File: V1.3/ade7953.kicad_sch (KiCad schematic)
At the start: 57 parts, among them U2 ADE7953xCP, Y1 3.58MHz

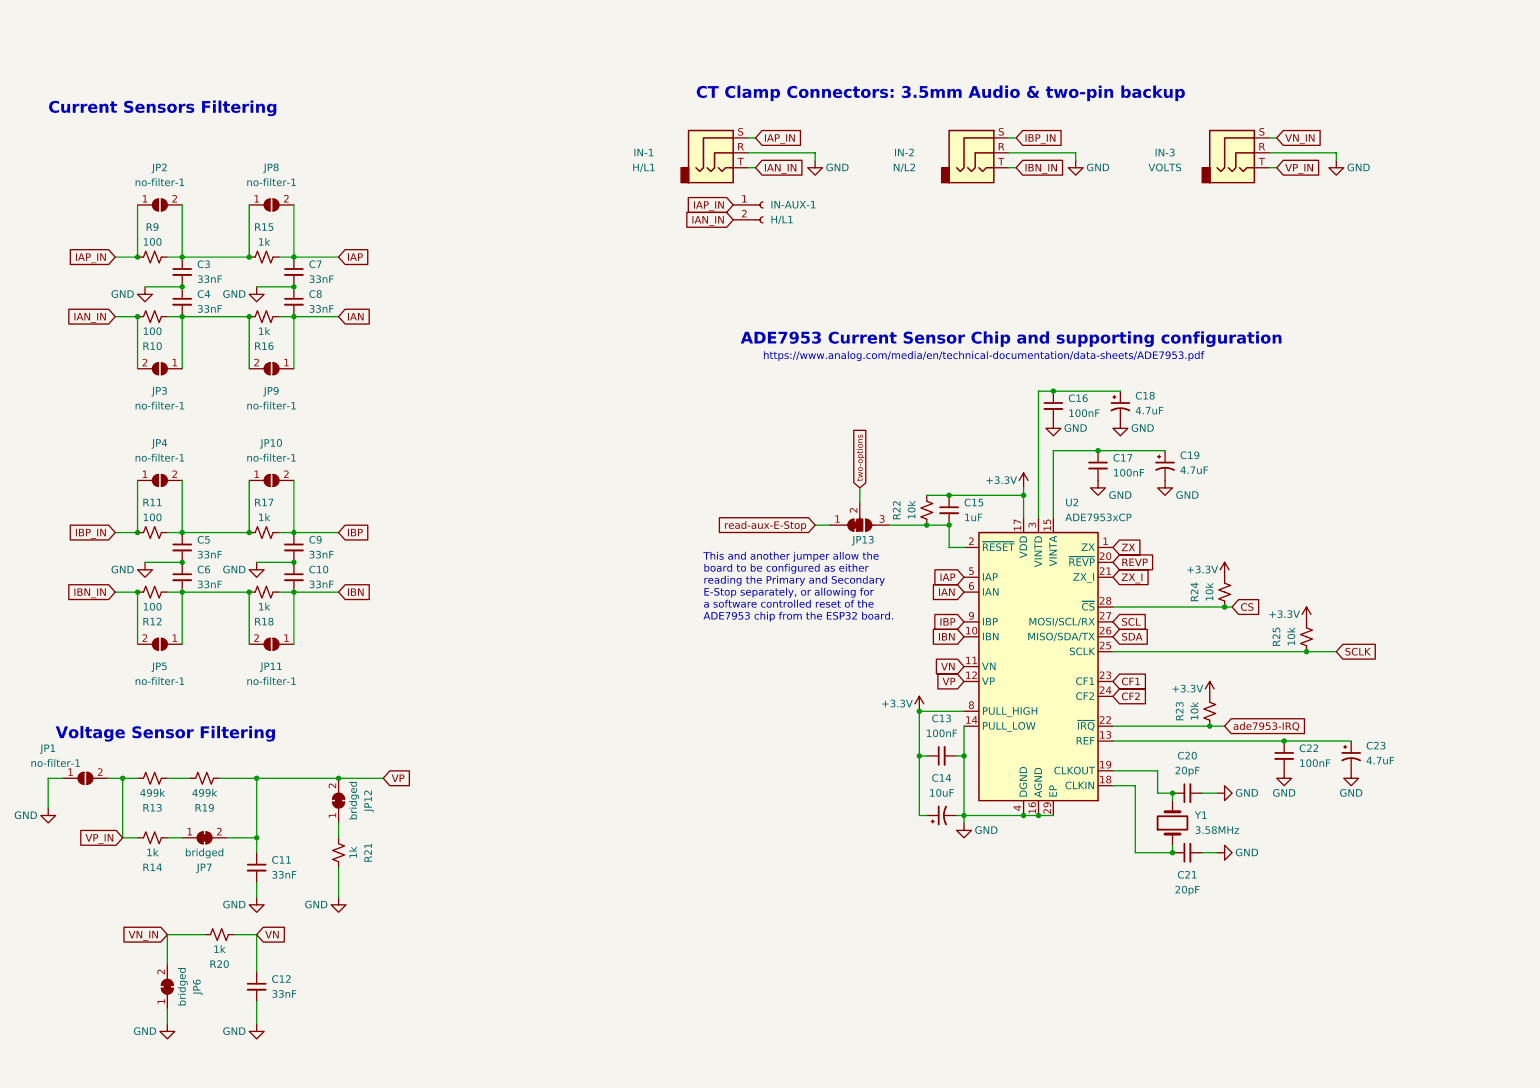
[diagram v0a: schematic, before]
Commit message: update v1.3 schematic documentation
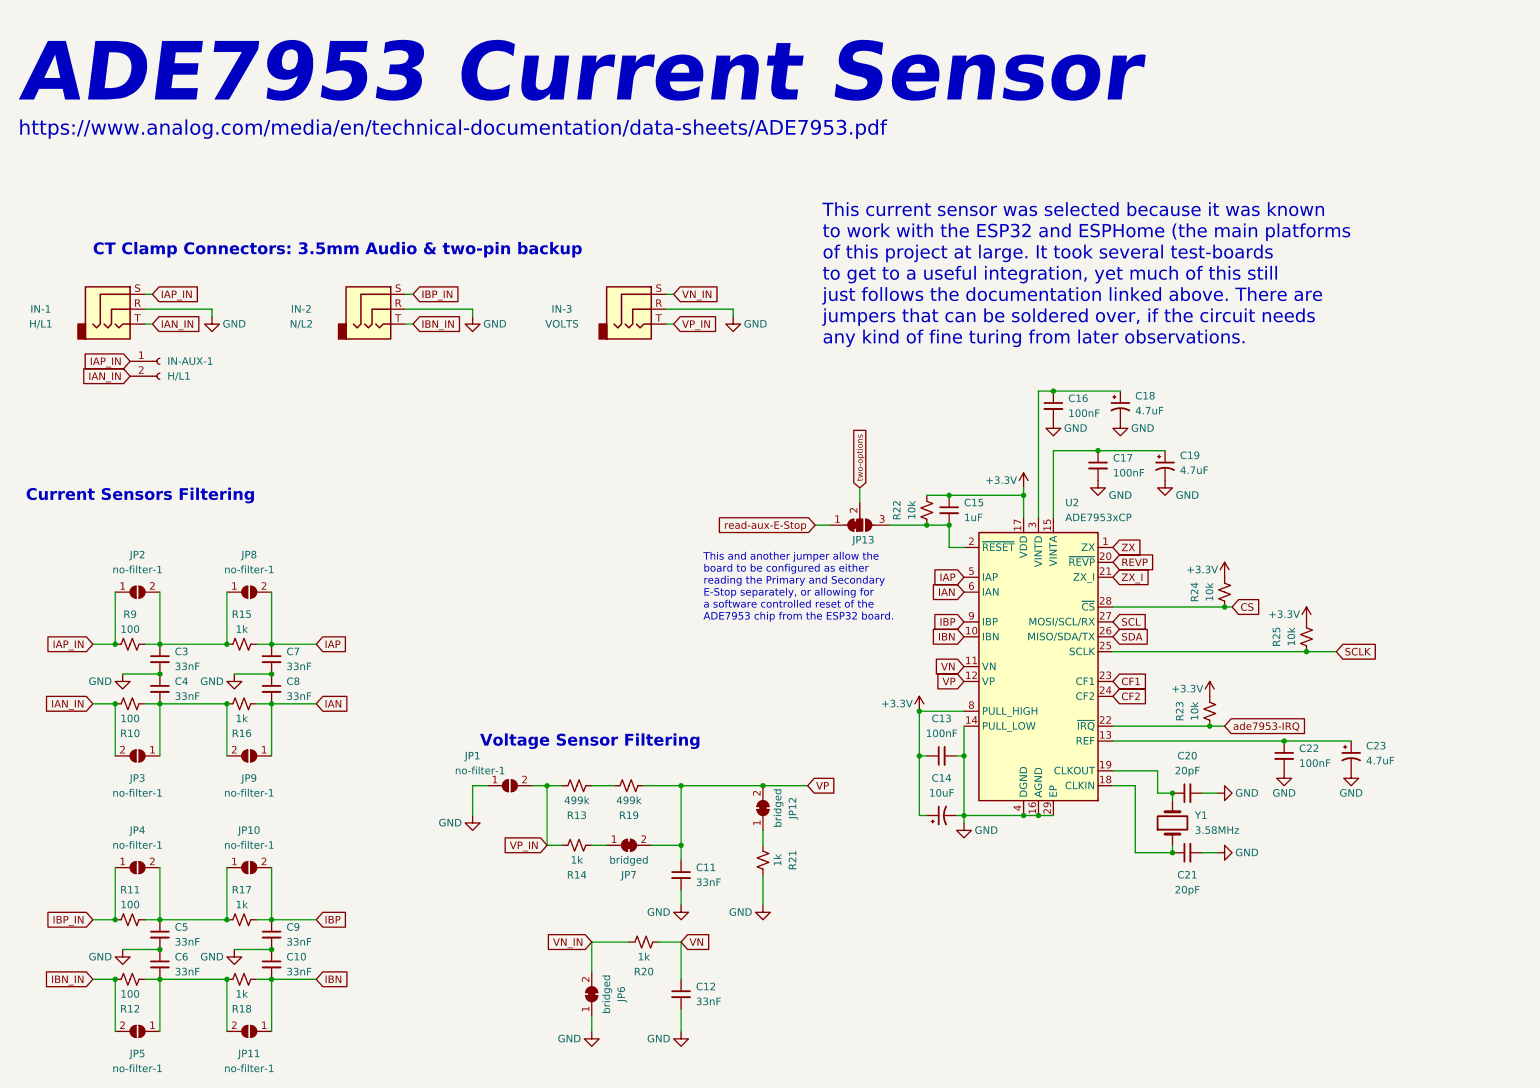
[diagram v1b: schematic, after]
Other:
- note added: "ADE7953 Current Sensor"
- note added: "This current sensor was selected because it was known to work with the ESP32 and ESPHome (the main platforms of this project at large. It took several test-boards to get to a useful integration, yet much of this still just follows the documentation linked above. There are jumpers that can be soldered over, if the circuit needs any kind of fine turing from later observations."
- note removed: "ADE7953 Current Sensor Chip and supporting configuration"
- moved on the sheet: C10, C11, C12, C3, C4, C5, C6, C7, C8, C9, IN-1, IN-2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
